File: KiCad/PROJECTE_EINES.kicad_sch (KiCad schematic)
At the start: 5 parts

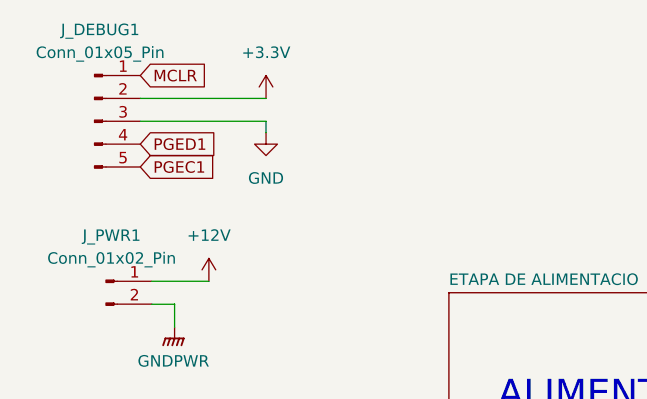
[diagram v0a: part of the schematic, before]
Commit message: V1 Routing
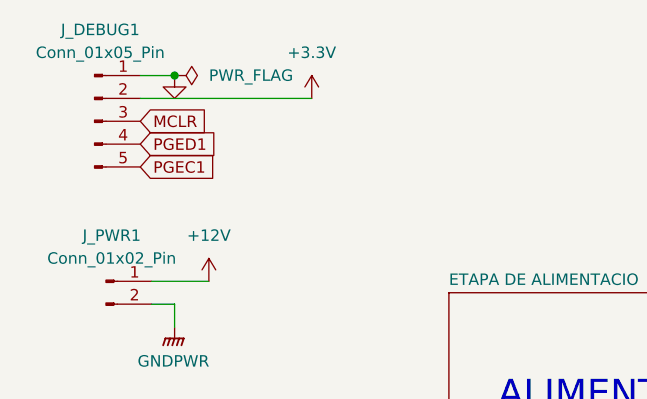
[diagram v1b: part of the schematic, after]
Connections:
- net GND: now also J_DEBUG1.1 (Pin_1); no longer J_DEBUG1.3 (Pin_3)
- net MCLR: now also J_DEBUG1.3 (Pin_3); no longer J_DEBUG1.1 (Pin_1)
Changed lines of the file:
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@@
+	)
+	(junction
+		(at 30.48 21.59)
+		(diameter 0)
+		(color 0 0 0 0)
 	)
 	(junction
@@
 	(wire
 		(pts
-			(xy 26.67 24.13) (xy 40.64 24.13)
+			(xy 26.67 24.13) (xy 45.72 24.13)
 		)
 		(stroke
@@
 	(wire
 		(pts
-			(xy 40.64 26.67) (xy 40.64 27.94)
+			(xy 20.32 93.98) (xy 22.86 93.98)
 		)
 		(stroke
@@
 	(wire
 		(pts
-			(xy 20.32 93.98) (xy 22.86 93.98)
+			(xy 20.32 95.25) (xy 20.32 93.98)
 		)
 		(stroke
@@
 	(wire
 		(pts
-			(xy 20.32 95.25) (xy 20.32 93.98)
+			(xy 26.67 21.59) (xy 30.48 21.59)
 		)
 		(stroke
@@
 	(wire
 		(pts
-			(xy 26.67 26.67) (xy 40.64 26.67)
+			(xy 43.18 95.25) (xy 43.18 93.98)
 		)
 		(stroke
@@
 	(wire
 		(pts
-			(xy 43.18 95.25) (xy 43.18 93.98)
+			(xy 30.48 46.99) (xy 30.48 49.53)
 		)
 		(stroke
@@
 	(wire
 		(pts
-			(xy 30.48 46.99) (xy 30.48 49.53)
+			(xy 22.86 93.98) (xy 27.94 93.98)
 		)
 		(stroke
@@
 		)
 	)
-	(wire
-		(pts
-			(xy 22.86 93.98) (xy 27.94 93.98)
-		)
-		(stroke
-			(width 0)
-			(type default)
-		)
-	)
 	(global_label "WIN_MOTOR_B"
 		(shape output)
@@
 	(global_label "MCLR"
 		(shape input)
-		(at 26.67 21.59 0)
-		(effects
-			(font
-				(size 1.27 1.27)
-			)
-			(justify left)
-		)
-		(property "Intersheetrefs" "${INTERSHEET_REFS}"
-			(at 26.67 21.59 0)
+		(at 26.67 26.67 0)
+		(effects
+			(font
+				(size 1.27 1.27)
+			)
+			(justify left)
+		)
+		(property "Intersheetrefs" "${INTERSHEET_REFS}"
+			(at 26.67 26.67 0)
 			(effects
 				(font
@@
 	(symbol
 		(lib_id "power:+3.3V")
-		(at 40.64 24.13 0)
+		(at 45.72 24.13 0)
 		(unit 1)
 		(exclude_from_sim no)
@@
 		(dnp no)
 		(fields_autoplaced yes)
-		(property "Reference" "#PWR03"
-			(at 40.64 27.94 0)
+		(property "Reference" "#PWR04"
+			(at 45.72 27.94 0)
 			(effects
 				(font
@@
 		)
 		(property "Value" "+3.3V"
-			(at 40.64 19.05 0)
+			(at 45.72 19.05 0)
 			(effects
 				(font
@@
 		)
 		(property "Footprint" ""
-			(at 40.64 24.13 0)
+			(at 45.72 24.13 0)
 			(effects
 				(font
@@
 		)
 		(property "Datasheet" ""
-			(at 40.64 24.13 0)
+			(at 45.72 24.13 0)
 			(effects
 				(font
@@
 		)
 		(property "Description" "Power symbol creates a global label with name \"+3.3V\""
-			(at 40.64 24.13 0)
+			(at 45.72 24.13 0)
 			(effects
 				(font
@@
 			(project ""
 				(path "/347831db-5db9-4aff-ad32-e56fd770e219"
-					(reference "#PWR03")
+					(reference "#PWR04")
 					(unit 1)
 				)
@@
 		(dnp no)
 		(fields_autoplaced yes)
-		(property "Reference" "#PWR05"
+		(property "Reference" "#PWR06"
 			(at 43.18 101.6 0)
 			(effects
@@
 			(project ""
 				(path "/347831db-5db9-4aff-ad32-e56fd770e219"
-					(reference "#PWR05")
+					(reference "#PWR06")
 					(unit 1)
 				)
@@
 	)
 	(symbol
+		(lib_id "power:PWR_FLAG")
+		(at 30.48 21.59 270)
+		(unit 1)
+		(exclude_from_sim no)
+		(in_bom yes)
+		(on_board yes)
+		(dnp no)
+		(fields_autoplaced yes)
+		(property "Reference" "#FLG07"
+			(at 32.385 21.59 0)
+			(effects
+				(font
+					(size 1.27 1.27)
+				)
+				(hide yes)
+			)
+		)
+		(property "Value" "PWR_FLAG"
+			(at 34.29 21.5899 90)
+			(effects
+				(font
+					(size 1.27 1.27)
+				)
+				(justify left)
+			)
+		)
+		(property "Footprint" ""
+			(at 30.48 21.59 0)
+			(effects
+				(font
+					(size 1.27 1.27)
+				)
+				(hide yes)
+			)
+		)
+		(property "Datasheet" "~"
+			(at 30.48 21.59 0)
+			(effects
+				(font
+					(size 1.27 1.27)
+				)
+				(hide yes)
+			)
+		)
+		(property "Description" "Special symbol for telling ERC where power comes from"
+			(at 30.48 21.59 0)
+			(effects
+				(font
+					(size 1.27 1.27)
+				)
+				(hide yes)
+			)
+		)
+		(pin "1"
+		)
+		(instances
+			(project ""
+				(path "/347831db-5db9-4aff-ad32-e56fd770e219"
+					(reference "#FLG07")
+					(unit 1)
+				)
+			)
+		)
+	)
+	(symbol
 		(lib_id "Connector:Conn_01x02_Pin")
 		(at 22.86 44.45 0)
@@
 		(dnp no)
 		(fields_autoplaced yes)
-		(property "Reference" "#PWR051"
+		(property "Reference" "#PWR03"
 			(at 34.29 48.26 0)
 			(effects
@@
 			(project "PROJECTE_EINES"
 				(path "/347831db-5db9-4aff-ad32-e56fd770e219"
-					(reference "#PWR051")
+					(reference "#PWR03")
 					(unit 1)
 				)
@@
 	(symbol
 		(lib_id "power:GND")
-		(at 40.64 27.94 0)
+		(at 30.48 21.59 0)
 		(unit 1)
 		(exclude_from_sim no)
@@
 		(dnp no)
 		(fields_autoplaced yes)
-		(property "Reference" "#PWR04"
-			(at 40.64 34.29 0)
+		(property "Reference" "#PWR05"
+			(at 30.48 27.94 0)
 			(effects
 				(font
@@
 		)
 		(property "Value" "GND"
-			(at 40.64 33.02 0)
-			(effects
-				(font
-					(size 1.27 1.27)
-				)
+			(at 30.48 26.67 0)
+			(effects
+				(font
+					(size 1.27 1.27)
+				)
+				(hide yes)
 			)
 		)
 		(property "Footprint" ""
-			(at 40.64 27.94 0)
+			(at 30.48 21.59 0)
 			(effects
 				(font
@@
 		)
 		(property "Datasheet" ""
-			(at 40.64 27.94 0)
+			(at 30.48 21.59 0)
 			(effects
 				(font
@@
 		)
 		(property "Description" "Power symbol creates a global label with name \"GND\" , ground"
-			(at 40.64 27.94 0)
+			(at 30.48 21.59 0)
 			(effects
 				(font
@@
 			(project "PROJECTE_EINES"
 				(path "/347831db-5db9-4aff-ad32-e56fd770e219"
-					(reference "#PWR04")
+					(reference "#PWR05")
 					(unit 1)
 				)
